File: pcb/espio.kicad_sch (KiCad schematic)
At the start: 27 parts, among them J1 Conn_Dbg_Header, J2 Conn_01x07, J3 Conn_01x08, J4 Conn_01x01, J5 Conn_01x08, J6 Conn_01x08, Q16 BC817, U1 MCP2562-E-SN, U5 LF50CPT-TR, U6 K776180WR-1

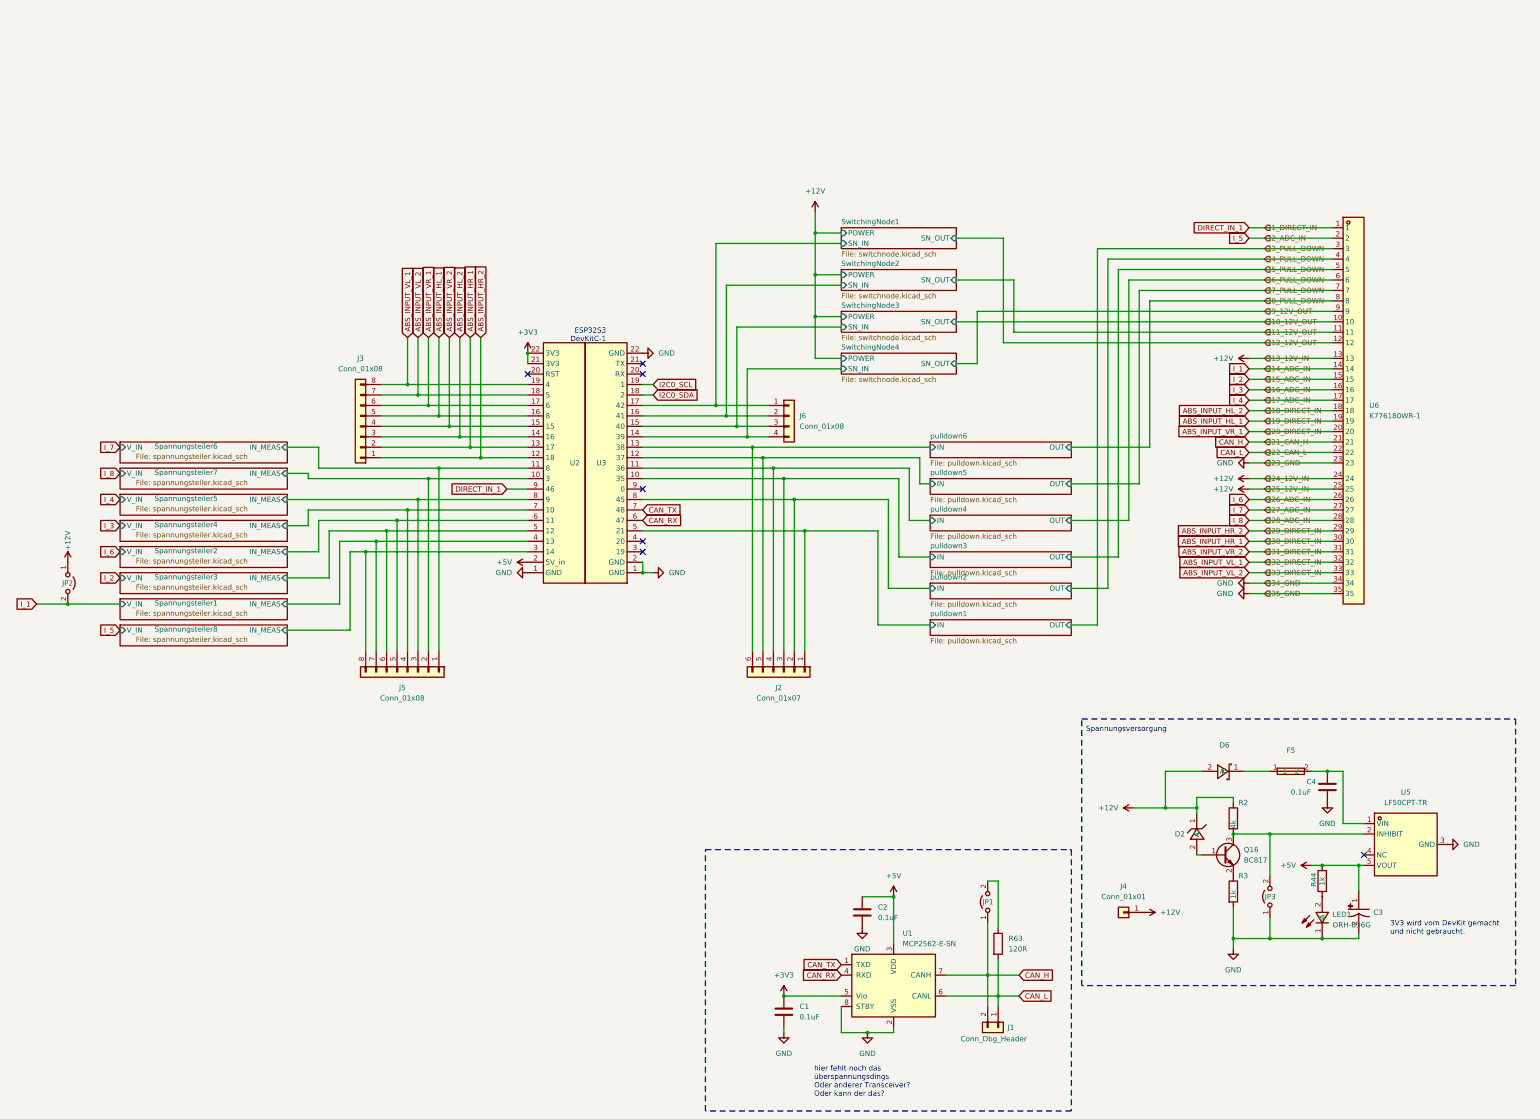
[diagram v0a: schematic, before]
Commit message: major work
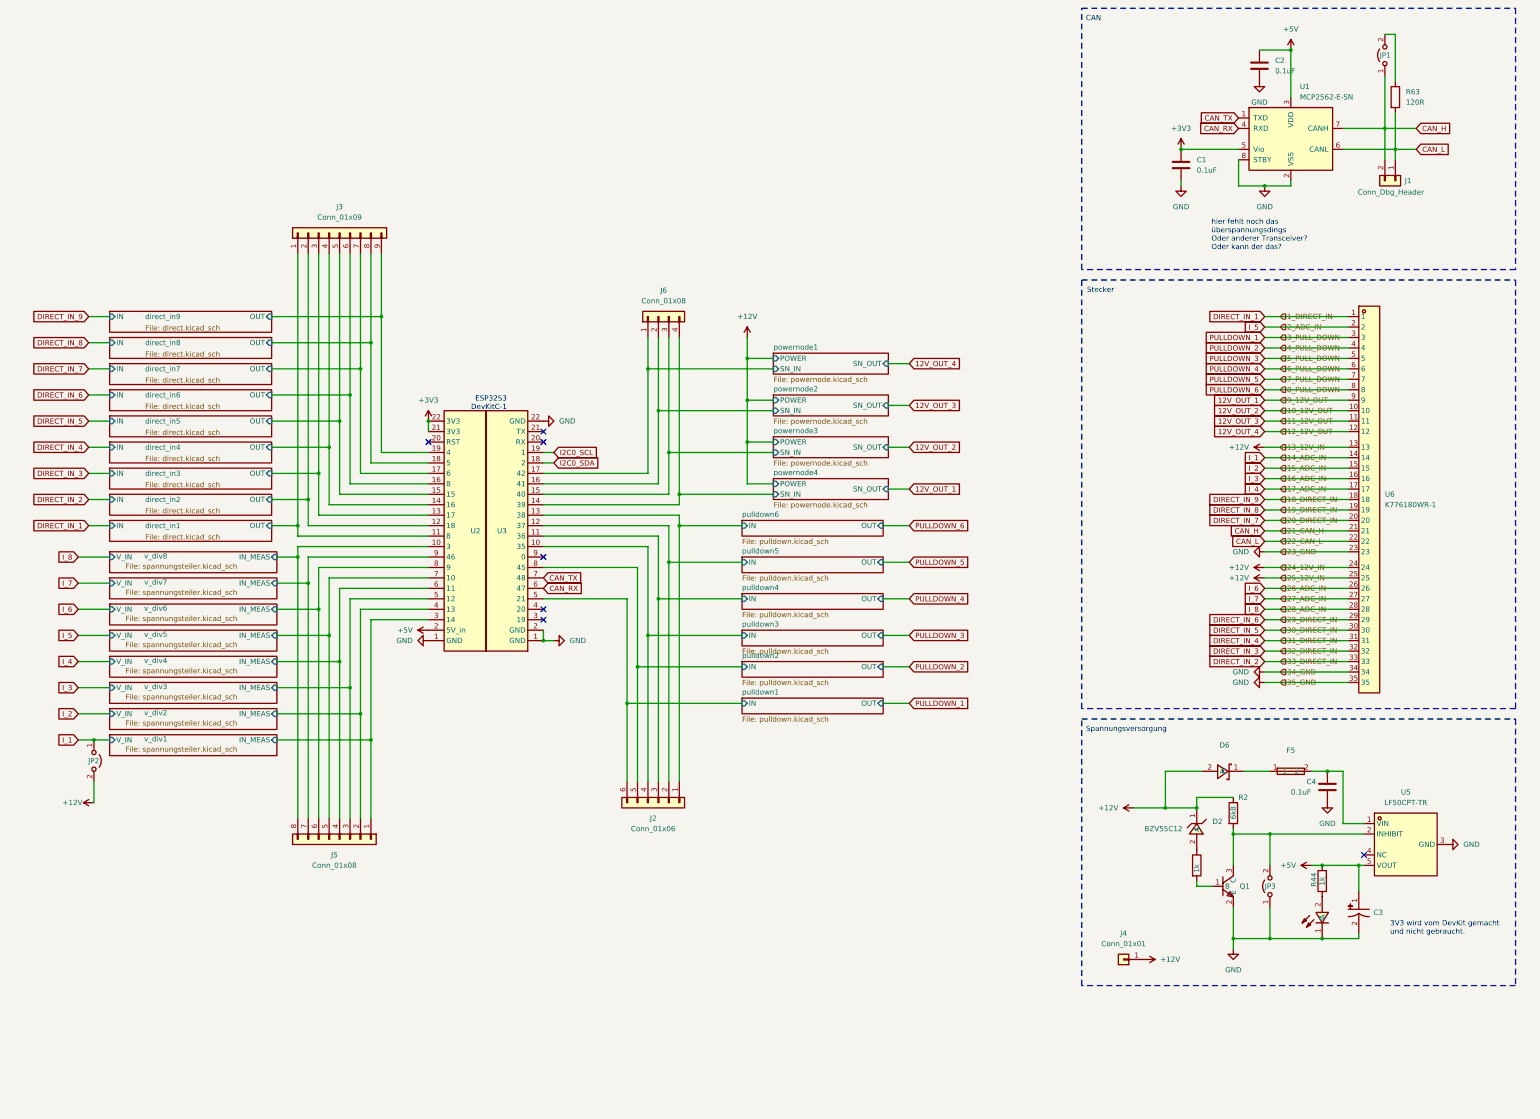
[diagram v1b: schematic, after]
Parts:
- removed D2: BZV55C15_C545332, lcsc:SOD-80_L3.5-W1.5-RD, symbol lcsc:BZV55C15_C545332
- removed Q16: BC817, Package_TO_SOT_SMD:SOT-23, symbol Transistor_BJT:BC817
- added D2: BZV55C12, lcsc:SOD-80_L3.5-W1.5-RD, symbol lcsc:BZV55C12
- added Q1: 2SC1623 300-400, lcsc:SOT-23-3_L2.9-W1.3-P1.90-LS2.4-BR, symbol lcsc:2SC1623300-400
- J2: value Conn_01x07 -> Conn_01x06
- J3: value Conn_01x08 -> Conn_01x09; footprint Connector_PinSocket_2.54mm:PinSocket_1x08_P2.54mm_Vertical -> Connector_PinSocket_2.54mm:PinSocket_1x09_P2.54mm_Vertical; symbol Connector_Generic:Conn_01x08 -> Connector_Generic:Conn_01x09; now in the parts list
- R2: value 4k -> 6k8
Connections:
- net +12V: now also JP2.2 (B), D2.1 (C); no longer JP2.1 (A)
- net DIRECT_IN_1: no longer U2.9 (46)
- net GND: now also Q1.2 (E); no longer R3.2
- net I_1: now also JP2.1 (A); no longer JP2.2 (B)
- net v_div1/IN_MEAS: now also J5.1 (Pin_1); no longer J5.8 (Pin_8)
- net pulldown1/IN: now also J2.6 (Pin_6); no longer J2.1 (Pin_1)
- net pulldown2/IN: now also J2.5 (Pin_5); no longer J2.2 (Pin_2)
- net pulldown3/IN: now also J2.4 (Pin_4); no longer J2.3 (Pin_3)
- net pulldown4/IN: now also J2.3 (Pin_3); no longer J2.4 (Pin_4)
- net pulldown5/IN: now also J2.2 (Pin_2); no longer J2.5 (Pin_5)
- net pulldown6/IN: now also J2.1 (Pin_1); no longer J2.6 (Pin_6)
- net at R3.1: now also D2.2 (A)
- net at JP3.2 (B), R2.2, U5.2 (INHIBIT): now also Q1.3 (C)
- net 10_12V_OUT renamed 12V_OUT_2
- net 11_12V_OUT renamed 12V_OUT_3
- net 12_12V_OUT renamed 12V_OUT_4
- net 3_PULL_DOWN renamed PULLDOWN_1
- net 4_PULL_DOWN renamed PULLDOWN_2
- net 5_PULL_DOWN renamed PULLDOWN_3
- net 6_PULL_DOWN renamed PULLDOWN_4
- net 7_PULL_DOWN renamed PULLDOWN_5
- net 8_PULL_DOWN renamed PULLDOWN_6
- net 9_12V_OUT renamed 12V_OUT_1
- removed net ABS_INPUT_HL_1: J3.5 (Pin_5), U2.16 (8), U6.19
- removed net ABS_INPUT_HL_2: J3.3 (Pin_3), U2.14 (16), U6.18
- removed net ABS_INPUT_HR_1: J3.2 (Pin_2), U2.13 (17), U6.30
- removed net ABS_INPUT_HR_2: J3.1 (Pin_1), U2.12 (18), U6.29
- removed net ABS_INPUT_VL_1: J3.8 (Pin_8), U2.19 (4), U6.32
- removed net ABS_INPUT_VL_2: J3.7 (Pin_7), U2.18 (5), U6.33
- removed net ABS_INPUT_VR_1: J3.6 (Pin_6), U2.17 (6), U6.20
- removed net ABS_INPUT_VR_2: J3.4 (Pin_4), U2.15, U6.31
- net Spannungsteiler1/IN_MEAS renamed v_div2/IN_MEAS
- net v_div2/IN_MEAS: now also J5.2 (Pin_2); no longer J5.7 (Pin_7)
- net Spannungsteiler2/IN_MEAS renamed v_div4/IN_MEAS
- net v_div4/IN_MEAS: now also J5.4 (Pin_4); no longer J5.5 (Pin_5)
- net Spannungsteiler3/IN_MEAS renamed v_div3/IN_MEAS
- net v_div3/IN_MEAS: now also J5.3 (Pin_3); no longer J5.6 (Pin_6)
- net Spannungsteiler4/IN_MEAS renamed v_div5/IN_MEAS
- net v_div5/IN_MEAS: now also J5.5 (Pin_5); no longer J5.4 (Pin_4)
- net Spannungsteiler5/IN_MEAS renamed v_div6/IN_MEAS
- net v_div6/IN_MEAS: now also J5.6 (Pin_6); no longer J5.3 (Pin_3)
- net Spannungsteiler6/IN_MEAS renamed direct_in1/OUT
- net direct_in1/OUT: now also J3.1 (Pin_1); no longer J5.1 (Pin_1)
- net Spannungsteiler7/IN_MEAS renamed v_div8/IN_MEAS
- net v_div8/IN_MEAS: now also J5.8 (Pin_8); no longer J5.2 (Pin_2)
- net SwitchingNode1/SN_IN renamed powernode1/SN_IN
- net SwitchingNode2/SN_IN renamed powernode2/SN_IN
- net SwitchingNode3/SN_IN renamed powernode3/SN_IN
- net SwitchingNode4/SN_IN renamed powernode4/SN_IN
- new net: Q1.1 (B), R3.2
- new net DIRECT_IN_2: U6.33
- new net DIRECT_IN_3: U6.32
- new net DIRECT_IN_4: U6.31
- new net DIRECT_IN_5: U6.30
- new net DIRECT_IN_6: U6.29
- new net DIRECT_IN_7: U6.20
- new net DIRECT_IN_8: U6.19
- new net DIRECT_IN_9: U6.18
- new net direct_in2/OUT: J3.2 (Pin_2), U2.12 (18)
- new net direct_in3/OUT: J3.3 (Pin_3), U2.13 (17)
- new net direct_in4/OUT: J3.4 (Pin_4), U2.14 (16)
- new net direct_in5/OUT: J3.5 (Pin_5), U2.15
- new net direct_in6/OUT: J3.6 (Pin_6), U2.16 (8)
- new net direct_in7/OUT: J3.7 (Pin_7), U2.17 (6)
- new net direct_in8/OUT: J3.8 (Pin_8), U2.18 (5)
- new net direct_in9/OUT: J3.9 (Pin_9), U2.19 (4)
- new net v_div7/IN_MEAS: J5.7 (Pin_7), U2.9 (46)
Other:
- sheet Spannungsteiler8 renamed v_div1
- removed sheet Spannungsteiler1
- removed sheet Spannungsteiler2
- removed sheet Spannungsteiler3
- removed sheet Spannungsteiler4
- removed sheet Spannungsteiler5
- removed sheet Spannungsteiler6
- removed sheet Spannungsteiler7
- removed sheet SwitchingNode1
- removed sheet SwitchingNode2
- removed sheet SwitchingNode3
- removed sheet SwitchingNode4
- added sheet direct_in1 (direct.kicad_sch)
- added sheet direct_in2 (direct.kicad_sch)
- added sheet direct_in3 (direct.kicad_sch)
- added sheet direct_in4 (direct.kicad_sch)
- added sheet direct_in5 (direct.kicad_sch)
- added sheet direct_in6 (direct.kicad_sch)
- added sheet direct_in7 (direct.kicad_sch)
- added sheet direct_in8 (direct.kicad_sch)
- added sheet direct_in9 (direct.kicad_sch)
- added sheet powernode1 (powernode.kicad_sch)
- added sheet powernode2 (powernode.kicad_sch)
- added sheet powernode3 (powernode.kicad_sch)
- added sheet powernode4 (powernode.kicad_sch)
- added sheet v_div2 (spannungsteiler.kicad_sch)
- added sheet v_div3 (spannungsteiler.kicad_sch)
- added sheet v_div4 (spannungsteiler.kicad_sch)
- added sheet v_div5 (spannungsteiler.kicad_sch)
- added sheet v_div6 (spannungsteiler.kicad_sch)
- added sheet v_div7 (spannungsteiler.kicad_sch)
- added sheet v_div8 (spannungsteiler.kicad_sch)
- note added: "CAN"
- note added: "Stecker"
- moved on the sheet: C1, C2, J1, J2, J4, J5, J6, JP1, JP2, JP3, R2, R63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
